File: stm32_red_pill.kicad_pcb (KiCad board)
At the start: 2 copper layers, 59 x 31 mm, 30 parts, among them J1 USB_B_Micro, J2 Conn_01x18, J3 Conn_01x18, J4 Conn_02x02_Top_Bottom, U1 STM32F103C8T6, U2 AMS1117-3.3, Y1 16MHZ

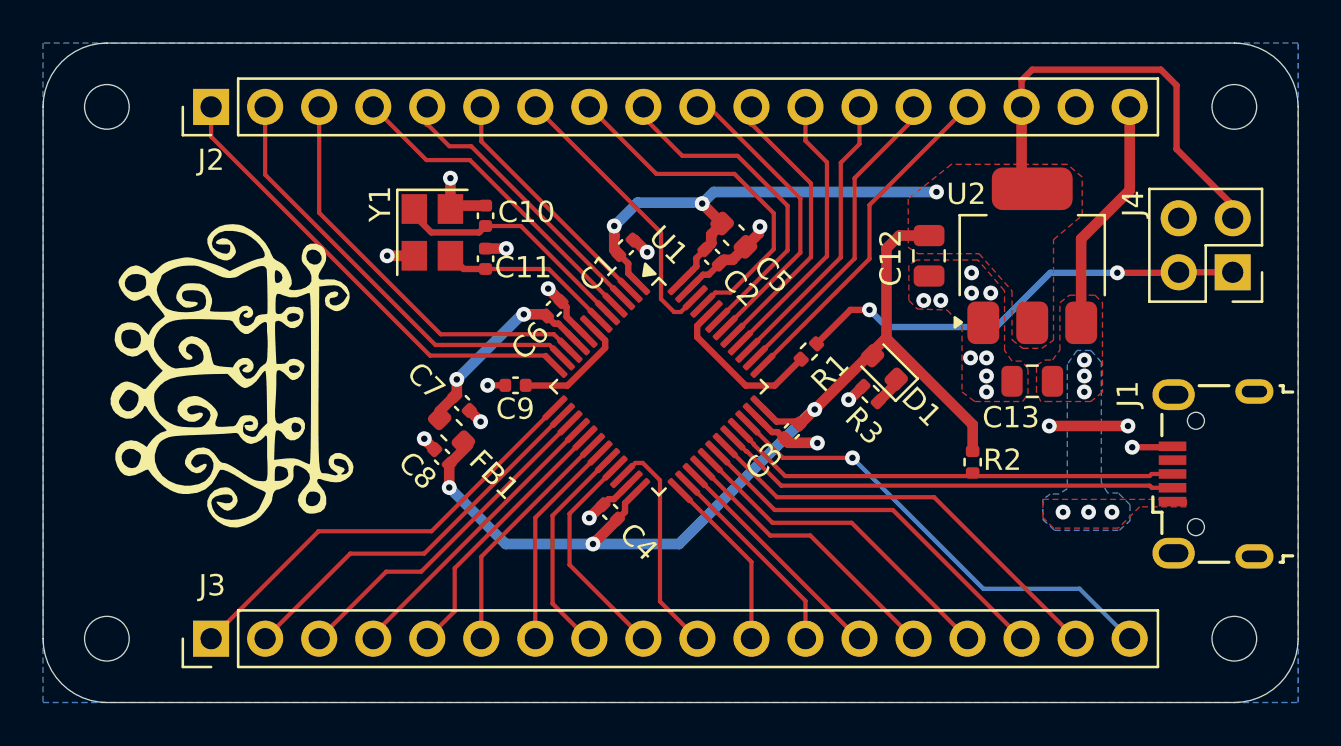
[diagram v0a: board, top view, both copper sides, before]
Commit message: update
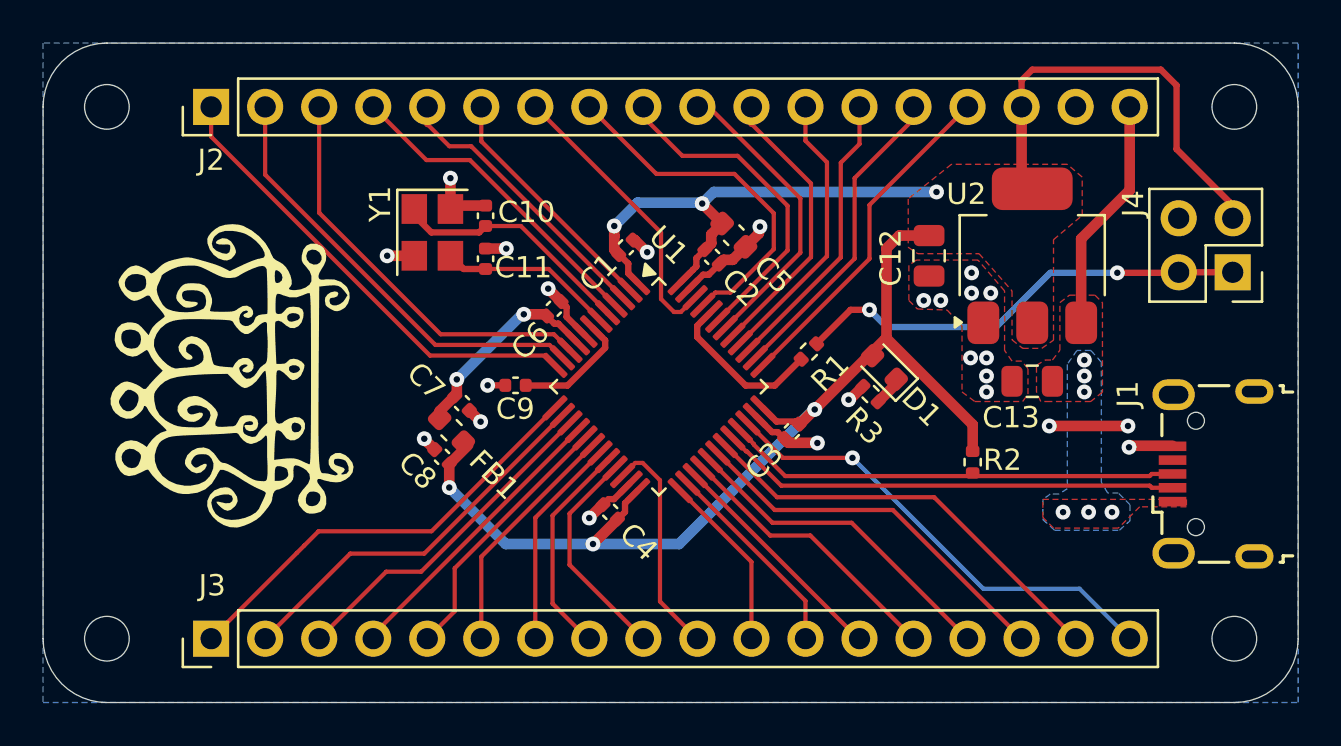
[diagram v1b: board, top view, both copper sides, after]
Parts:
- D1: value BLUE -> RED
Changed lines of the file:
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@@
 			)
 		)
-		(property "MPN" "C1691"
+		(property "MPN" "C19702"
 			(at 0 0 315)
 			(unlocked yes)
@@
 			)
 		)
-		(property "MPN" "C14445"
+		(property "MPN" "C52923"
 			(at 0 0 315)
 			(unlocked yes)
@@
 			)
 		)
-		(property "MPN" "C25531"
+		(property "MPN" "C25744"
 			(at 0 0 225)
 			(unlocked yes)
@@
 			)
 		)
-		(property "MPN" "C5674"
+		(property "MPN" "C45783"
 			(at 0 0 270)
 			(unlocked yes)
@@
 			)
 		)
-		(property "MPN" "C5674"
+		(property "MPN" "C45783"
 			(at 0 0 180)
 			(unlocked yes)
@@
 			)
 		)
-		(property "Value" "BLUE"
+		(property "Value" "RED"
 			(at 0 1.43 135)
 			(layer "F.Fab")
@@
 			)
 		)
-		(property "MPN" "C2288"
+		(property "MPN" "C2286"
 			(at 0 0 135)
 			(unlocked yes)
@@
 			)
 		)
-		(property "MPN" "C14445"
+		(property "MPN" "C52923"
 			(at 0 0 135)
 			(unlocked yes)
@@
 	)
 	(segment
-		(start 114.271391 104.289411)
-		(end 114.531767 104.289411)
+		(start 133.05 105)
+		(end 133.095 104.955)
 		(width 0.3)
 		(layer "F.Cu")
@@
 	)
 	(segment
-		(start 131.2 105)
-		(end 133.05 105)
+		(start 114.271391 104.289411)
+		(end 114.531767 104.289411)
 		(width 0.3)
 		(layer "F.Cu")
@@
 	)
 	(segment
-		(start 133.05 105)
-		(end 133.095 104.955)
-		(width 0.3)
-		(layer "F.Cu")
-		(net 2)
-	)
-	(segment
 		(start 106.581767 107.439411)
 		(end 106.321178 107.7)
@@
 	)
 	(segment
+		(start 131.121 104.929)
+		(end 133.095 104.929)
+		(width 0.5)
+		(layer "F.Cu")
+		(net 2)
+	)
+	(segment
 		(start 101.775 95.66)
 		(end 100.8 95.66)
@@
 	)
 	(segment
+		(start 131.05 105)
+		(end 131.121 104.929)
+		(width 0.5)
+		(layer "F.Cu")
+		(net 2)
+	)
+	(segment
 		(start 116.4 104.8)
 		(end 116.389411 104.789411)
@@
 	)
 	(via
-		(at 131.2 105)
+		(at 131.05 105)
 		(size 0.7)
 		(drill 0.3)
@@
 	)
 	(segment
-		(start 92.95 108.95)
-		(end 87.9 114)
+		(start 92.278075 109.621925)
+		(end 91.929889 109.970111)
+		(width 0.2)
+		(layer "F.Cu")
+		(net 35)
+	)
+	(segment
+		(start 98.260912 108.95)
+		(end 92.95 108.95)
 		(width 0.2)
 		(layer "F.Cu")
@@
 	)
 	(segment
-		(start 98.260912 108.95)
-		(end 92.95 108.95)
+		(start 92.95 108.95)
+		(end 92.278075 109.621925)
+		(width 0.2)
+		(layer "F.Cu")
+		(net 35)
+	)
+	(segment
+		(start 91.929889 109.970111)
+		(end 87.9 114)
 		(width 0.2)
 		(layer "F.Cu")
@@
 		)
 	)
+	(generated
+		(type tuning_pattern)
+		(name "Tuning Pattern")
+		(layer "F.Cu")
+		(base_line
+			(pts
+				(xy 92.278075 109.621925) (xy 91.929889 109.970111)
+			)
+		)
+		(corner_radius_percent 80)
+		(end
+			(xy 91.929889 109.970111)
+		)
+		(initial_side "right")
+		(last_diff_pair_gap 0.18)
+		(last_netname "/PA3")
+		(last_status "tuned")
+		(last_track_width 0.2)
+		(last_tuning "20,6568 mm (afgestemd)")
+		(max_amplitude 1)
+		(min_amplitude 0.2)
+		(min_spacing 0.6)
+		(origin
+			(xy 92.278075 109.621925)
+		)
+		(override_custom_rules no)
+		(rounded yes)
+		(single_sided no)
+		(target_length 1000000)
+		(target_length_max 1000000)
+		(target_length_min 0)
+		(target_skew 0)
+		(target_skew_max 0.1)
+		(target_skew_min -0.1)
+		(tuning_mode "single")
+		(members "2fa81aa1-0389-46ab-8d65-f9b8b98f6ecb")
+	)
 	(embedded_fonts no)
